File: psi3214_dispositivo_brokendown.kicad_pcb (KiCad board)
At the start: 2 copper layers, 51.5 x 67 mm, 25 parts, among them J2 AudioJack3, J4 Conn_01x03, J5 AudioJack3, U1 TL072_sim, U2 MAX1044

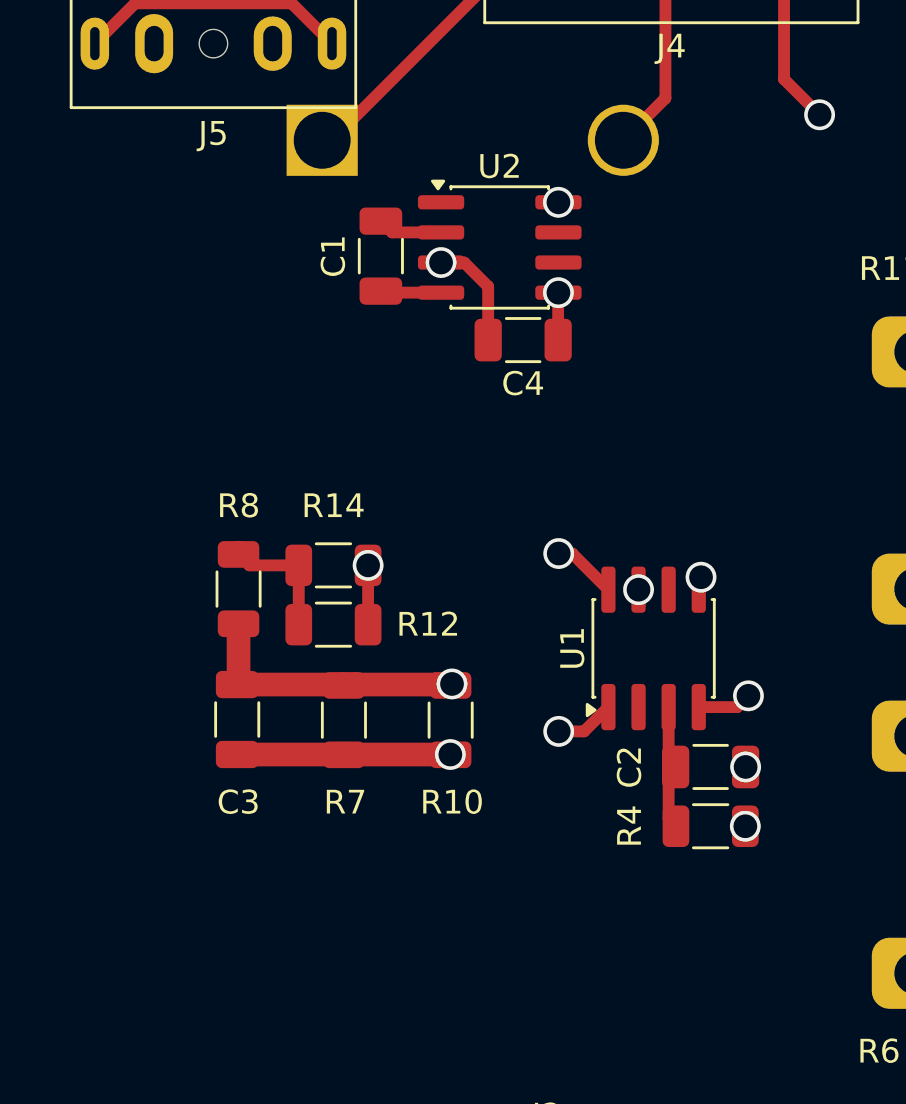
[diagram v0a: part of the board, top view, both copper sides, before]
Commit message: Got it
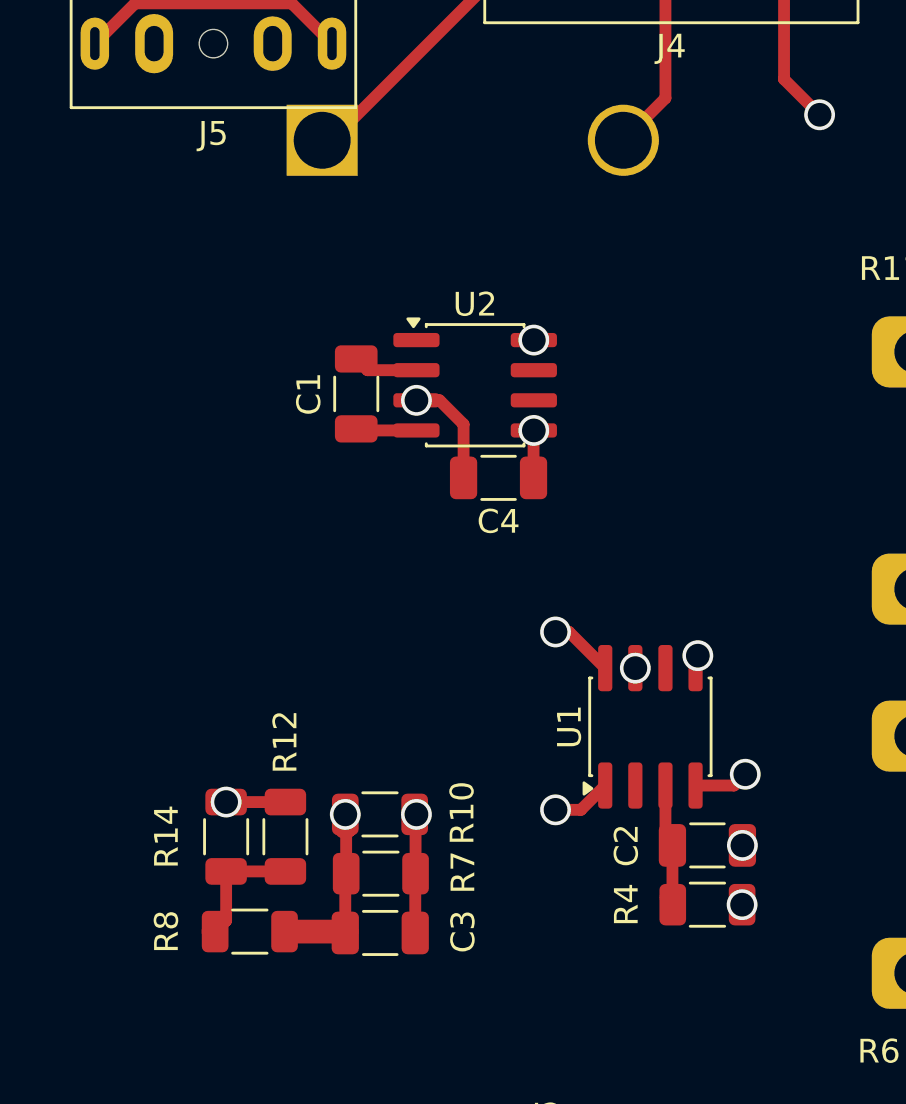
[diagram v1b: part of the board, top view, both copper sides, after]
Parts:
- moved R8 14.5 mm to (141.5, 114.4), turned to 0 degrees
- moved R14 12.3 mm to (140.5, 110.4), turned to -90 degrees
- moved C3 10.8 mm to (147.0, 114.5), turned to 180 degrees
- moved R12 9.17 mm to (143.0, 110.4), turned to -90 degrees
- moved R7 6.66 mm to (147.0, 112.0), turned to 180 degrees
- moved C1 5.90 mm to (146.0, 91.8)
- moved C4 5.90 mm to (152.0, 95.3)
- moved U2 5.90 mm to (151.0, 91.4)
- moved R10 4.97 mm to (147.0, 109.5), turned to 180 degrees
- moved C2 3.31 mm to (160.8, 110.8)
- moved R4 3.31 mm to (160.8, 113.3)
- moved U1 3.31 mm to (158.4, 105.8)
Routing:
- net saida_filtro: track 12.4 -> 8.22 mm
- net saida_amp1: track 11.5 -> 7.54 mm
